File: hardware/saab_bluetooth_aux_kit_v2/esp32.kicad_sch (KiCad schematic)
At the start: 2 parts, among them U1 ESP32_30Pin_Breakout, U2 WeMos_LoLin32_Lite

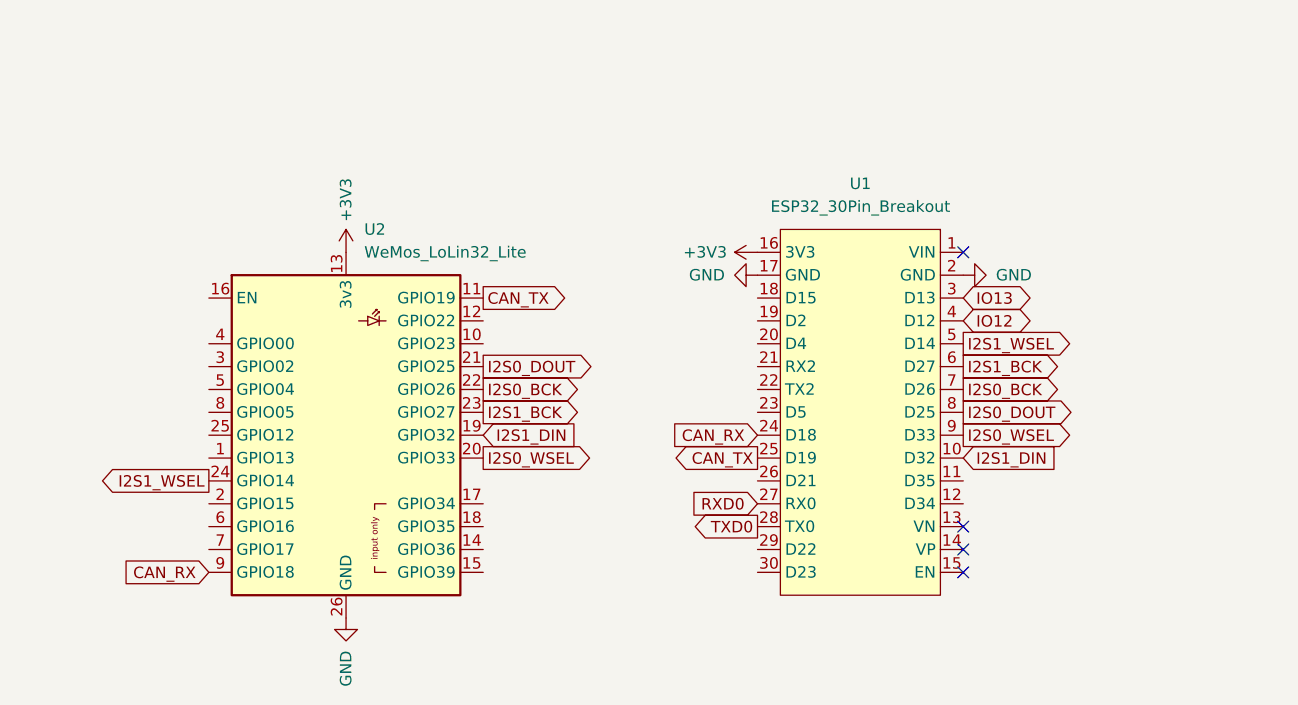
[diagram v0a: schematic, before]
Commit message: V2 Kit looking good!
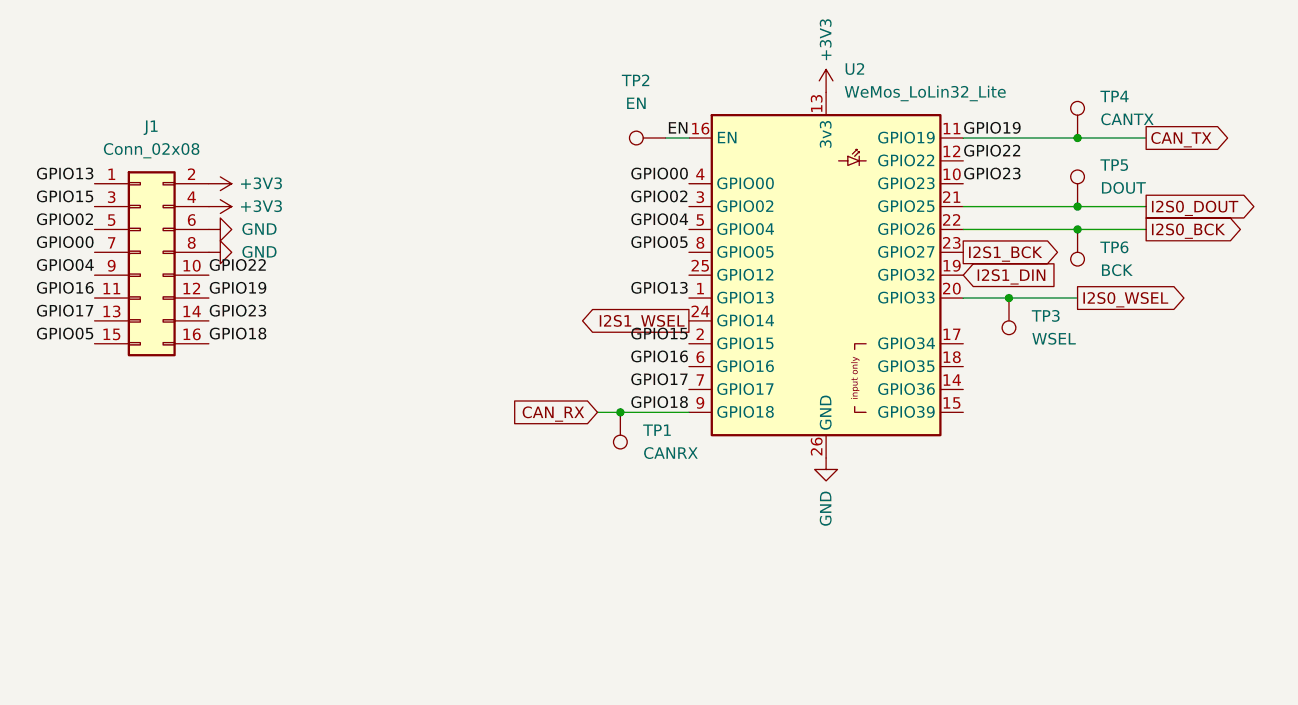
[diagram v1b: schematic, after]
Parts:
- removed U1: ESP32_30Pin_Breakout, kicadlibrary:ESP32_30Pin_Breakout, symbol esp32_30pin_breakout:ESP32_30Pin_Breakout
- added J1: Conn_02x08, Connector_PinHeader_2.54mm:PinHeader_2x08_P2.54mm_Vertical, symbol Connector_Generic:Conn_02x08_Odd_Even
- added TP1: CANRX, TestPoint:TestPoint_THTPad_D2.0mm_Drill1.0mm, symbol Connector:TestPoint
- added TP2: EN, TestPoint:TestPoint_THTPad_D2.0mm_Drill1.0mm, symbol Connector:TestPoint
- added TP3: WSEL, TestPoint:TestPoint_THTPad_D2.0mm_Drill1.0mm, symbol Connector:TestPoint
- added TP4: CANTX, TestPoint:TestPoint_THTPad_D2.0mm_Drill1.0mm, symbol Connector:TestPoint
- added TP5: DOUT, TestPoint:TestPoint_THTPad_D2.0mm_Drill1.0mm, symbol Connector:TestPoint
- added TP6: BCK, TestPoint:TestPoint_THTPad_D2.0mm_Drill1.0mm, symbol Connector:TestPoint
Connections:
- net +3V3: now also J1.2 (Pin_2), J1.4 (Pin_4)
- net CAN_RX: now also J1.16 (Pin_16), TP1.1
- net CAN_TX: now also J1.12 (Pin_12), TP4.1
- net GND: now also J1.6 (Pin_6), J1.8 (Pin_8)
- net I2S0_BCK: now also TP6.1
- net I2S0_DOUT: now also TP5.1
- net I2S0_WSEL: now also TP3.1
- net GPIO13: now reaches U2.1 (GPIO13)
- net GPIO13: now also J1.1 (Pin_1)
- net GPIO23: now reaches U2.10 (GPIO23)
- net GPIO23: now also J1.14 (Pin_14)
- net GPIO22: now reaches U2.12 (GPIO22)
- net GPIO22: now also J1.10 (Pin_10)
- net EN: now reaches U2.16 (EN)
- net EN: now also TP2.1
- net GPIO15: now reaches U2.2 (GPIO15)
- net GPIO15: now also J1.3 (Pin_3)
- net GPIO02: now reaches U2.3 (GPIO02)
- net GPIO02: now also J1.5 (Pin_5)
- net GPIO00: now reaches U2.4 (GPIO00)
- net GPIO00: now also J1.7 (Pin_7)
- net GPIO04: now reaches U2.5 (GPIO04)
- net GPIO04: now also J1.9 (Pin_9)
- net GPIO16: now reaches U2.6 (GPIO16)
- net GPIO16: now also J1.11 (Pin_11)
- net GPIO17: now reaches U2.7 (GPIO17)
- net GPIO17: now also J1.13 (Pin_13)
- net GPIO05: now reaches U2.8 (GPIO05)
- net GPIO05: now also J1.15 (Pin_15)
- no-connect marks 4 -> 0
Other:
- moved on the sheet: U2
